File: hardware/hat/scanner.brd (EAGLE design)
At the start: 65 x 56 mm, 24 parts, among them U1 CAT24C32WI-GT3, U2 TPS61165DBV

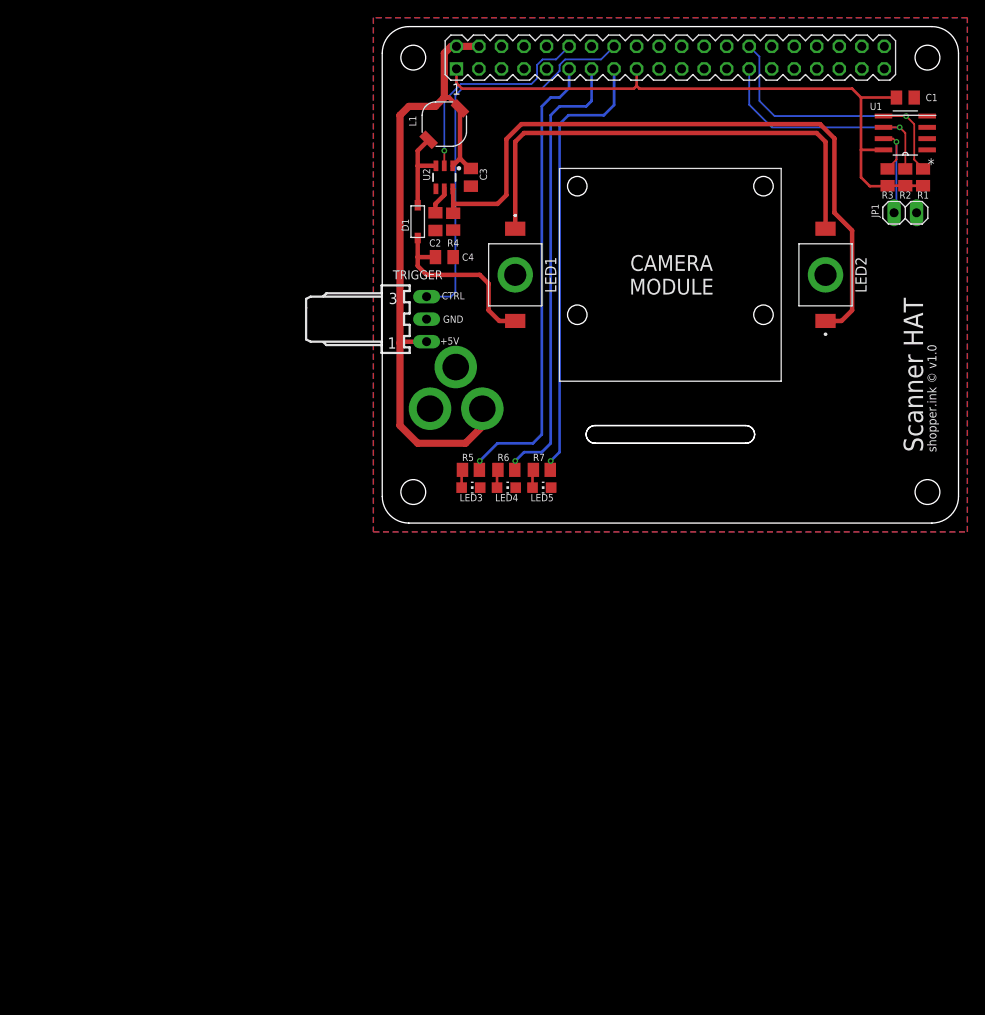
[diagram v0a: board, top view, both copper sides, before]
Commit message: fixed issues with 1.0
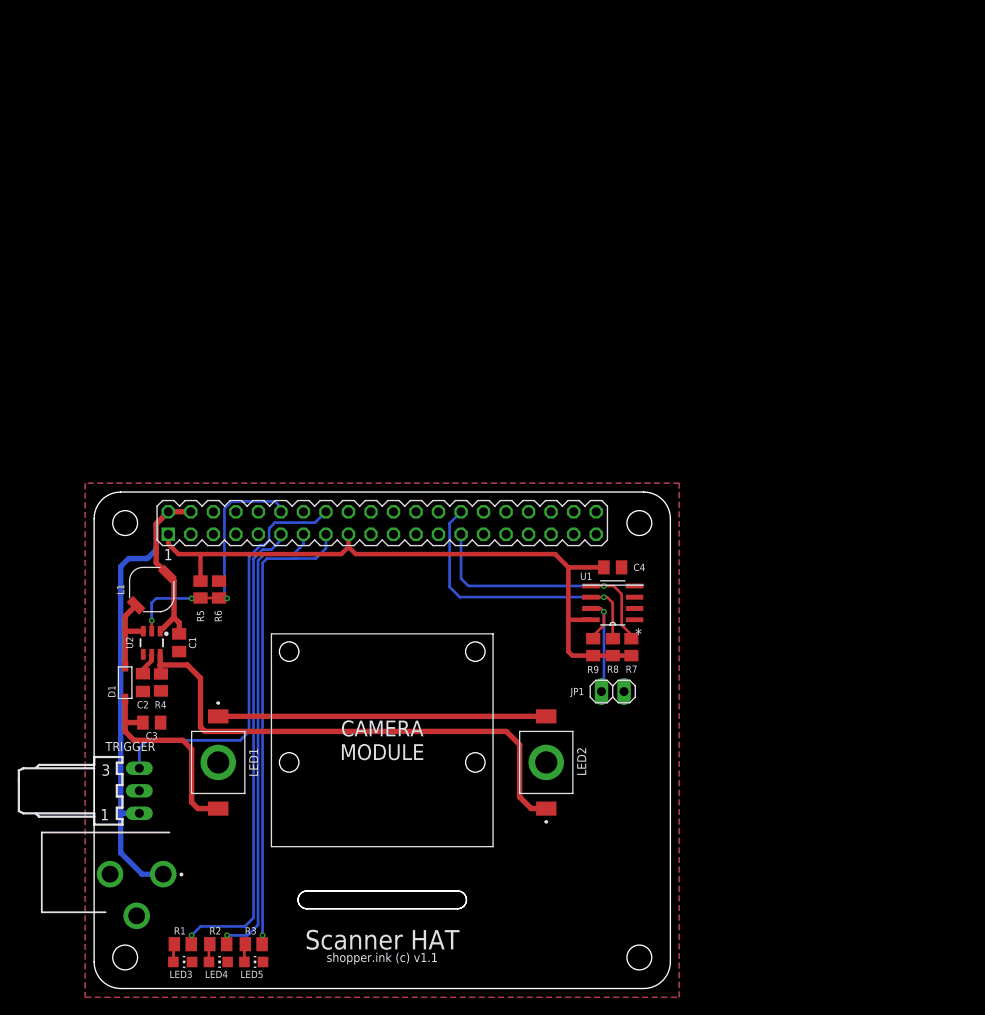
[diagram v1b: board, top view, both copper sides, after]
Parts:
- added R8, R9: 3k9, resistor:M0805
- C1: value 100nF -> 4.7μF
- C3: value 4.7μF -> 1μF
- C4: value 1μF -> 100nF
- POWER: value 2.1MMJACKTHM -> PJ-102AH; device adafruit:PJ-102A -> PJ-102AH:PJ-102AH
- R1, R2: value 3k9 -> 330
- R3: value 3k9 -> 10k
- R5, R6: value 330 -> (none)
- R7: value 10k -> 3k9
- moved R1 120.2 mm to (-22.5, -47.5), turned to 180 degrees
- moved R2 116.1 mm to (-18.5, -47.5), turned to 180 degrees
- moved R3 112.2 mm to (-14.5, -47.5), turned to 180 degrees
- moved C1 102.4 mm to (-22.9, -13.5), turned to 270 degrees
- moved C3 71.3 mm to (-26.0, -22.5), turned to 0 degrees
- moved LED1 64.4 mm to (-18.5, -27.0)
- moved POWER 64.2 mm to (-27.7, -43.9), flipped to the top, turned to 90 degrees
- moved LED2 63.4 mm to (18.5, -27.0)
- moved JP1 63.3 mm to (26.0, -19.0)
- moved LED3 62.6 mm to (-22.5, -49.5)
- moved LED4 62.6 mm to (-18.5, -49.5)
- moved LED5 62.6 mm to (-14.5, -49.5)
- moved U1 62.4 mm to (26.0, -9.00)
- moved TRIGGER 62.3 mm to (-27.4, -30.2)
- moved L1 62.0 mm to (-26.0, -7.50)
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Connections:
- net N$7 renamed LED_COMP
- removed net N$10: C4.1, D1.C, LED1.2
- new net N$2: C3.1, D1.C, LED1.2
- net +3V3: now also C4.1, R5.2, R7.2, R8.2, R9.1; no longer C1.1, R1.2, R2.2, R3.1
- net +5V: now also C1.1, POWER.1; no longer C3.1, POWER.TIP
- net EEPROM_SCL: now also GPIO.28, R8.1; no longer GPIO.27, R2.1
- net EEPROM_SDA: now also GPIO.27, R7.1; no longer GPIO.28, R1.1
- net EEPROM_WP: now also R9.2; no longer R3.2
- net GND: now also POWER.2, POWER.3, R6.1; no longer POWER.RING, POWER.RING_SW
- net LED3: now also R1.1; no longer R5.1
- net LED4: now also R2.1; no longer R6.1
- net LED5: now also R3.1; no longer R7.1
- net LED_CTRL: now also R5.1, R6.2
- net N$13: now also R1.2; no longer R5.2
- net N$17: now also R2.2; no longer R6.2
- net N$18: now also R3.2; no longer R7.2
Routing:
- net N$2: track 0.00 -> 23.3 mm
- net N$10: track 20.5 -> 0.00 mm
- net N$3: track 55.4 -> 37.0 mm
- net LED_FB: track 77.6 -> 59.2 mm
- net +5V: track 76.8 -> 70.0 mm
- net LED_CTRL: track 24.8 -> 29.7 mm, vias 1 -> 3
- net EEPROM_SCL: track 28.8 -> 33.7 mm
- net +3V3: track 73.1 -> 75.8 mm
- net EEPROM_SDA: track 33.2 -> 30.8 mm
- net LED5: track 50.6 -> 52.4 mm
- net LED3: track 52.4 -> 53.9 mm
- net LED4: track 51.7 -> 53.1 mm
- net EEPROM_WP: track 13.2 -> 14.3 mm
- net LED_COMP: track 3.11 -> 2.61 mm
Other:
- board text added: "shopper.ink (c) v1.1"
- board text removed: "+5V"
- board text removed: "CTRL"
- board text removed: "GND"
- board text removed: "shopper.ink © v1.0"
